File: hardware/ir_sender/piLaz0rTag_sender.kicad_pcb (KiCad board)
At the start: 2 copper layers, 18.2 x 17.2 mm, 3 parts

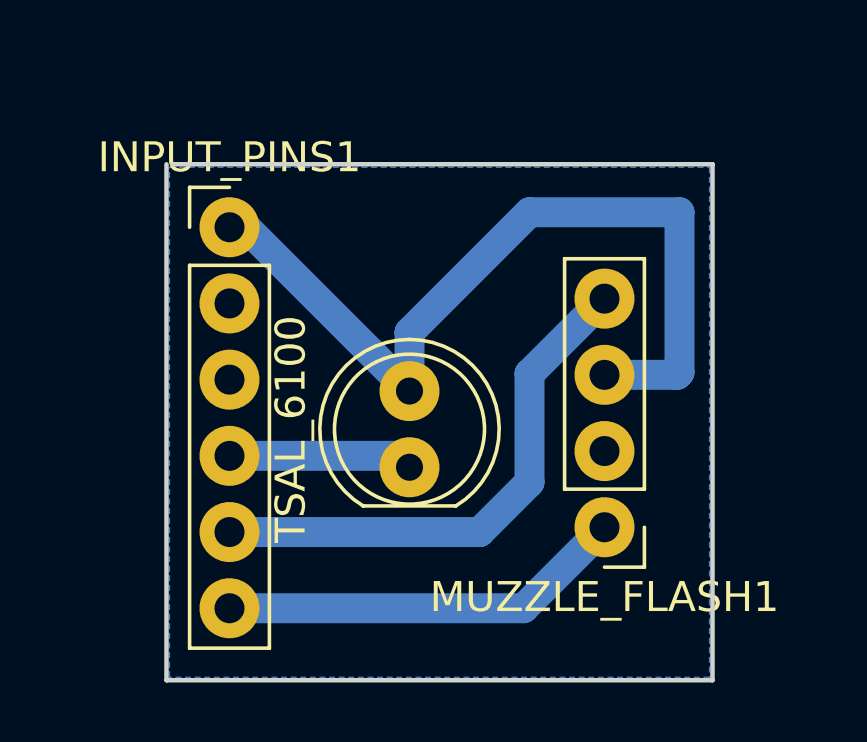
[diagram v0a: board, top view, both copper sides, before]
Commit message: Some new sender gerber stuff
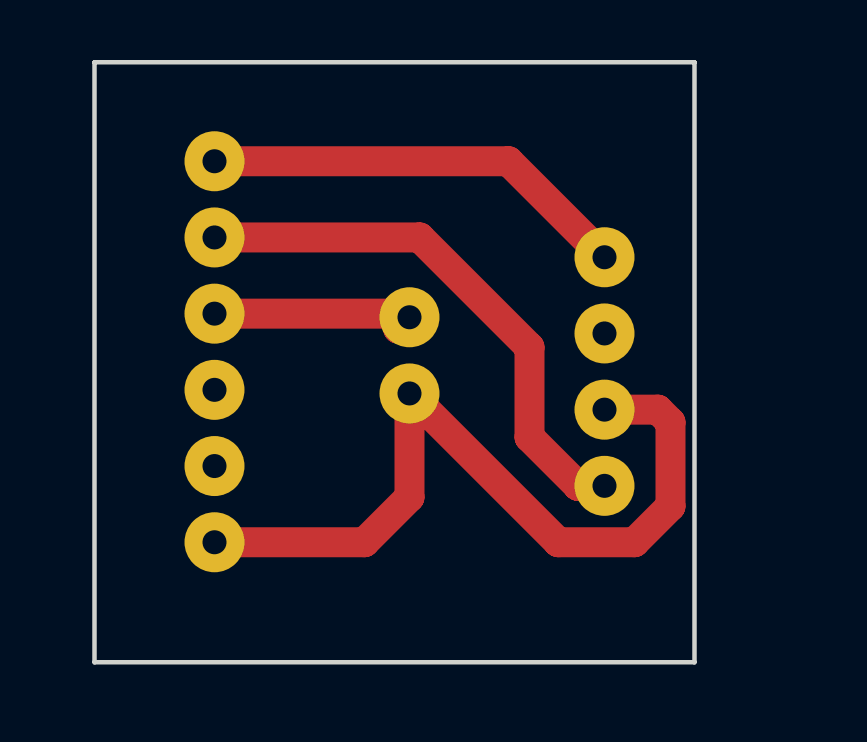
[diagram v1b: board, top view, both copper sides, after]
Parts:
- INPUT_PINS1, MUZZLE_FLASH1, TSAL_6100: moved to B.Cu
- moved INPUT_PINS1 10.5 mm to (141.0, 111.0)
- moved MUZZLE_FLASH1 9.00 mm to (154.0, 101.5)
- moved TSAL_6100 5.00 mm to (147.5, 103.5), turned to 270 degrees
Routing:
- net +5V: track 29.2 -> 27.5 mm
- net Net-(INPUT_PINS1-Pad5): track 17.8 -> 19.1 mm
- net /IR_LED_ON: track 6.69 -> 7.62 mm
- net Net-(INPUT_PINS1-Pad6): track 13.6 -> 14.3 mm
- added copper zone on F.Cu, net GND
- removed copper zone on B.Cu, net GND
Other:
- board size 18.2 x 17.2 mm -> 20 x 20 mm
